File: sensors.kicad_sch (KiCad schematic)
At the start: 11 parts, among them J4 Conn_01x05_Pin, U12 CY15B064J-SXET, U3 MMC5983MA, U4 BMI088, U9 MCP23009-E/MG

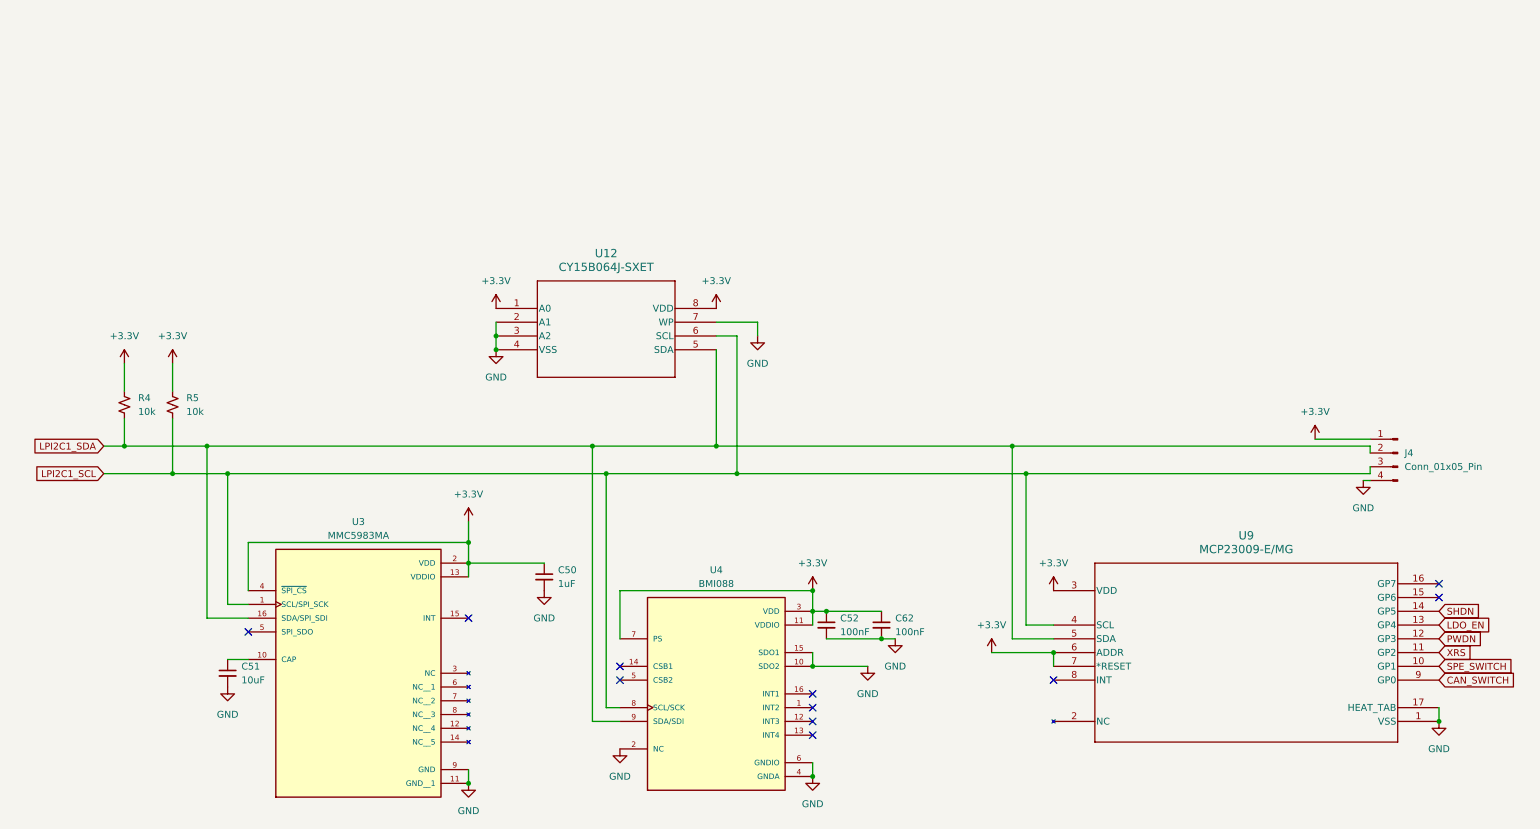
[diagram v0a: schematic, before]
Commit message: v0.2
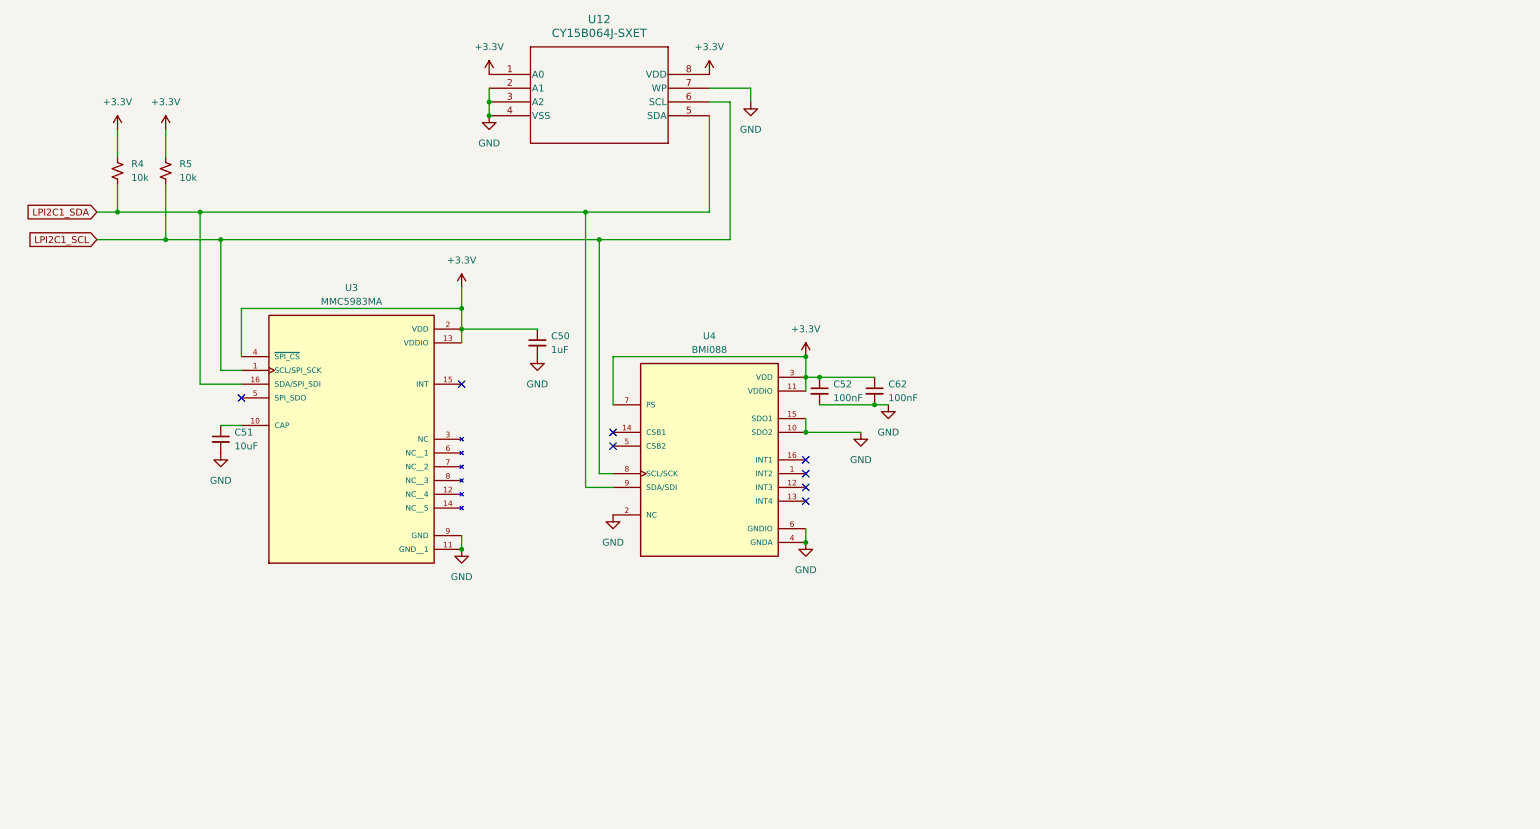
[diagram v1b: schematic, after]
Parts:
- removed J4: Conn_01x05_Pin, Connector_PinHeader_2.00mm:PinHeader_1x04_P2.00mm_Vertical, symbol Connector:Conn_01x04_Pin
- removed U9: MCP23009-E/MG, QFN16_3x3MC_MCH, symbol MCP23009-E:MCP23009-E_MG
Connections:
- no-connect marks 11 -> 8
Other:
- title: RT1050 DevBoard for Project Horizon -> Payload Board for Pleiades Atlas
- moved on the sheet: C50, C51, C52, C62, R4, R5, U12, U3, U4
